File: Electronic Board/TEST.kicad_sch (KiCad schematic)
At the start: 54 parts, among them J1_guitare_entrée1 NRJ6HF, J2 4840.2201, J2_guitare_sortie1 NRJ6HF, J3 173950578, SW2 SW_SPDT, U1 LM7805_TO220, U2 BU18SD2MG-MTR, U4 SGTL5000XNAA3, U5 IS42S16400J-xC

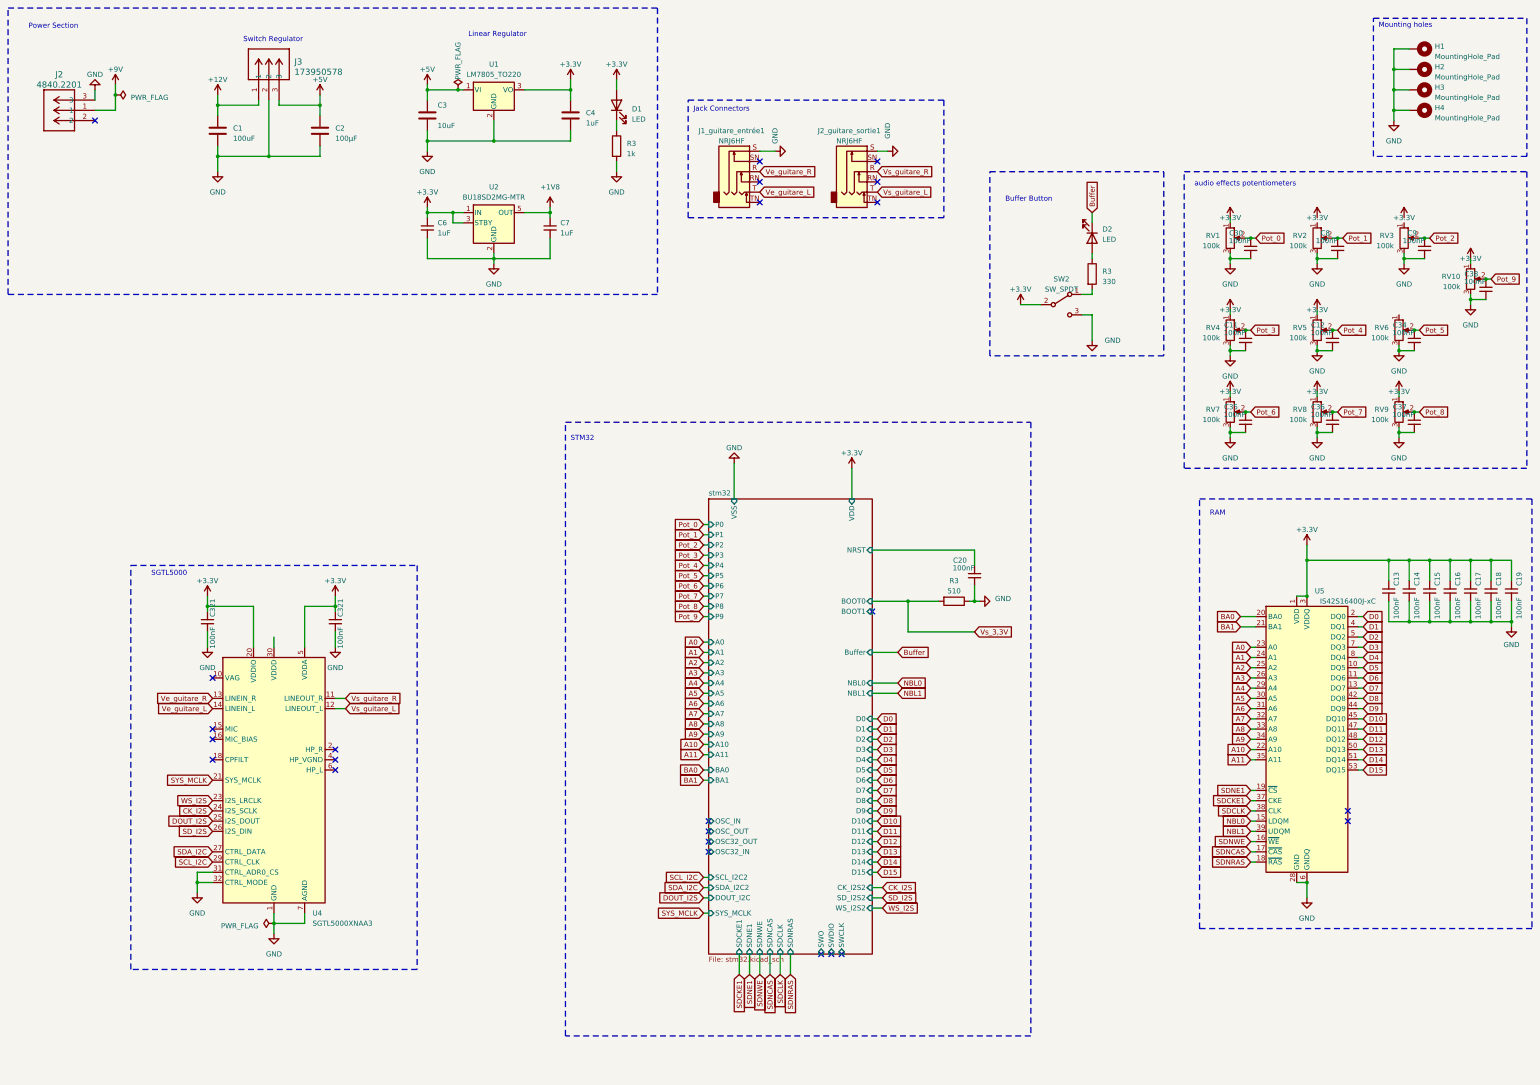
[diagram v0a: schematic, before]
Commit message: Add files via upload
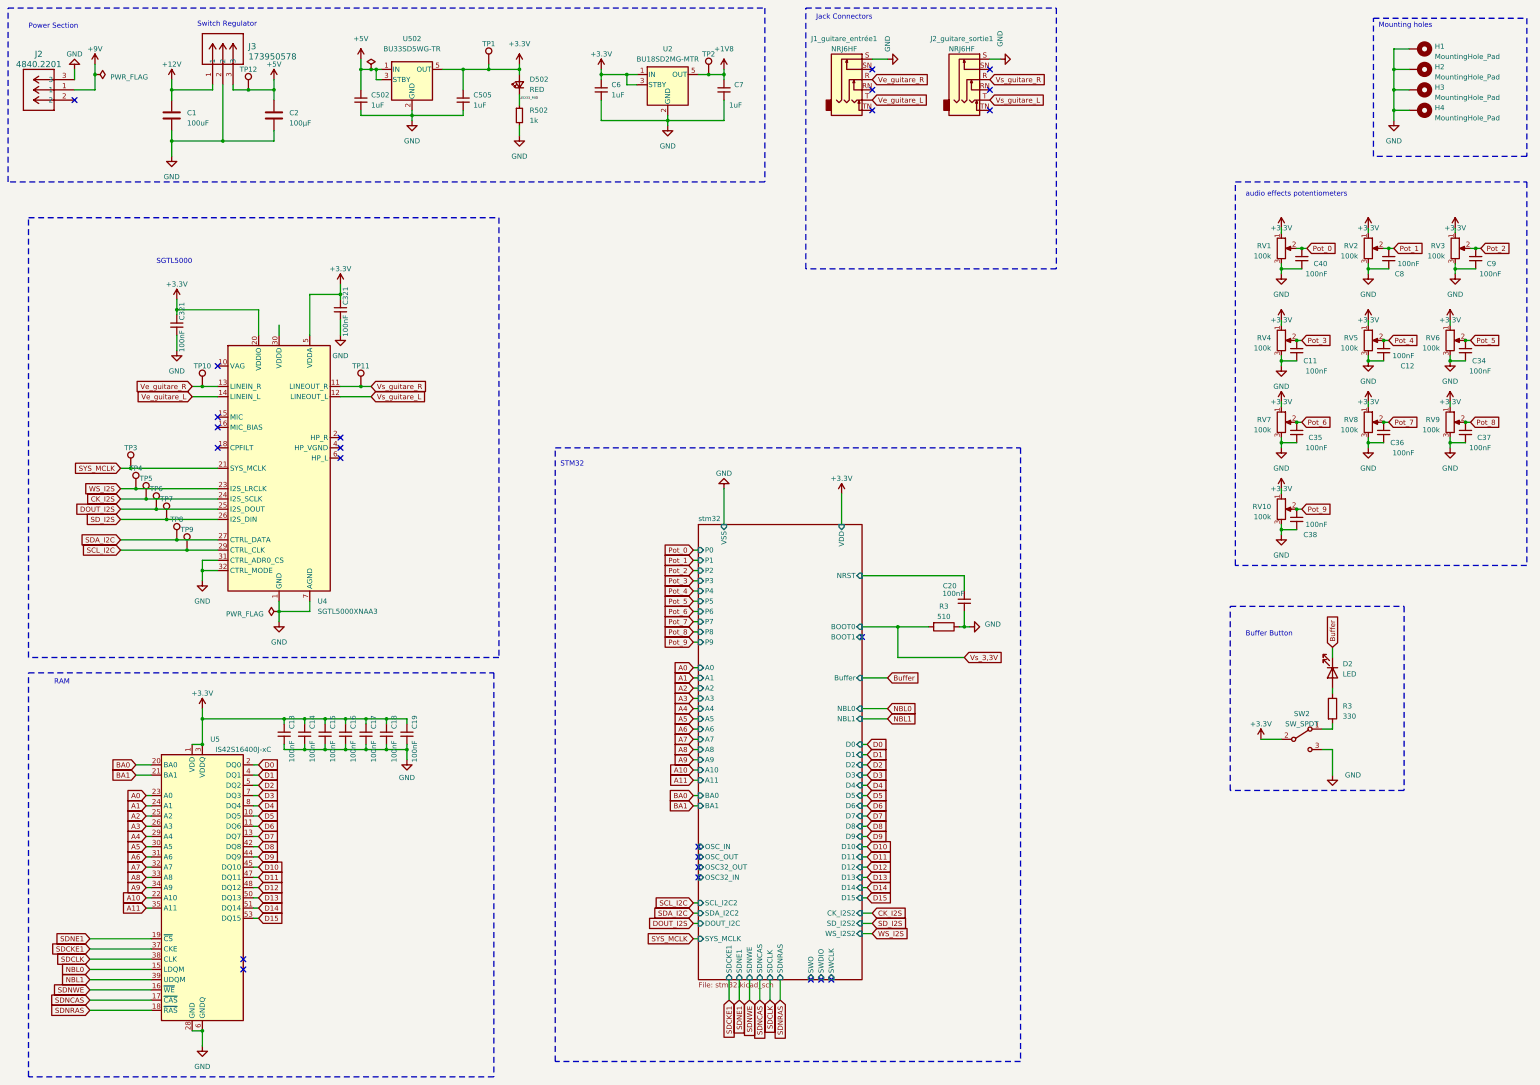
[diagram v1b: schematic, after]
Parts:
- removed C3: 10uF, Capacitor_SMD:C_0201_0603Metric_Pad0.64x0.40mm_HandSolder, symbol Device:C
- removed C4: 1uF, Capacitor_SMD:C_0201_0603Metric_Pad0.64x0.40mm_HandSolder, symbol Device:C
- removed D1: LED, LED_SMD:LED_0201_0603Metric_Pad0.64x0.40mm_HandSolder, symbol Device:LED
- removed R3: 1k, Resistor_SMD:R_0201_0603Metric_Pad0.64x0.40mm_HandSolder, symbol Device:R
- removed U1: LM7805_TO220, Package_TO_SOT_THT:TO-220-3_Vertical, symbol Regulator_Linear:LM7805_TO220
- added C502, C505: 1uF, Capacitor_SMD:C_0603_1608Metric, symbol Device:C_Small
- added D502: RED, LED_SMD:LED_0603_1608Metric, symbol Device:LED_Small
- added R502: 1k, Resistor_SMD:R_0603_1608Metric, symbol Device:R_Small
- added TP1, TP10, TP11, TP12, TP2, TP3, TP4, TP5, TP6, TP7, TP8, TP9: TestPoint, TestPoint:TestPoint_Pad_D1.5mm, symbol Connector:TestPoint
- added U502: BU33SD5WG-TR, Package_TO_SOT_SMD:SOT-23-5, symbol WITNS_ROHM:BU33SD5WG-TR
- renumbered C30 to C40
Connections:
- net +1V8: now also TP2.1
- net +3.3V: now also RV2.1, RV3.1, RV6.1, C505.1, D502.2 (A), TP1.1, U502.5 (OUT)
- net +5V: now also C502.1, TP12.1, U502.1 (IN), U502.3 (STBY)
- net CK_I2S: now also TP5.1
- net DOUT_I2S: now also TP6.1
- net GND: now also C502.2, C505.2, R502.2, U502.2 (GND)
- net SCL_I2C: now also TP9.1
- net SDA_I2C: now also TP8.1
- net SD_I2S: now also TP7.1
- net SYS_MCLK: now also TP3.1
- net Ve_guitare_R: now also TP10.1
- net Vs_guitare_R: now also TP11.1
- net WS_I2S: now also TP4.1
- new net LED33_MID: D502.1 (K), R502.1
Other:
- note removed: "Linear Regulator"
- moved on the sheet: C1, C11, C12, C13, C14, C15, C16, C17, C18, C19, C2, C20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
